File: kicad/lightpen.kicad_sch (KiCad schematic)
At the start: 4 parts, among them J16 Light Pen, U141 74LS74, U89 74LS04

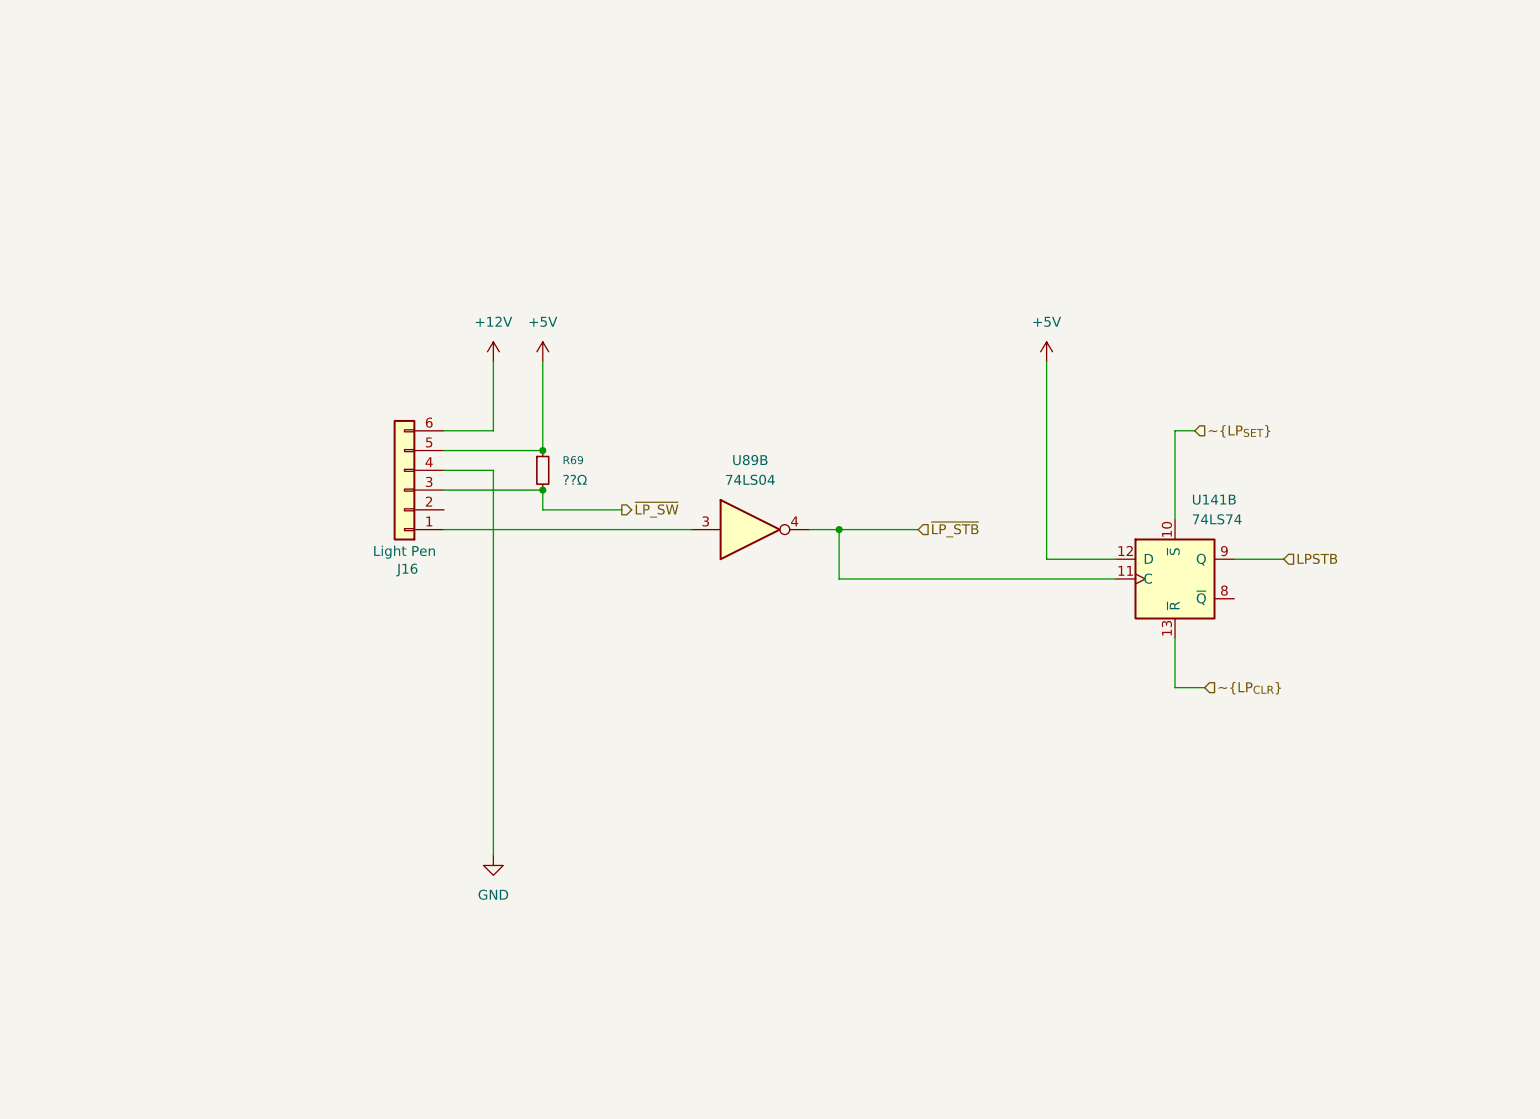
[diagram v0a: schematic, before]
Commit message: More updates
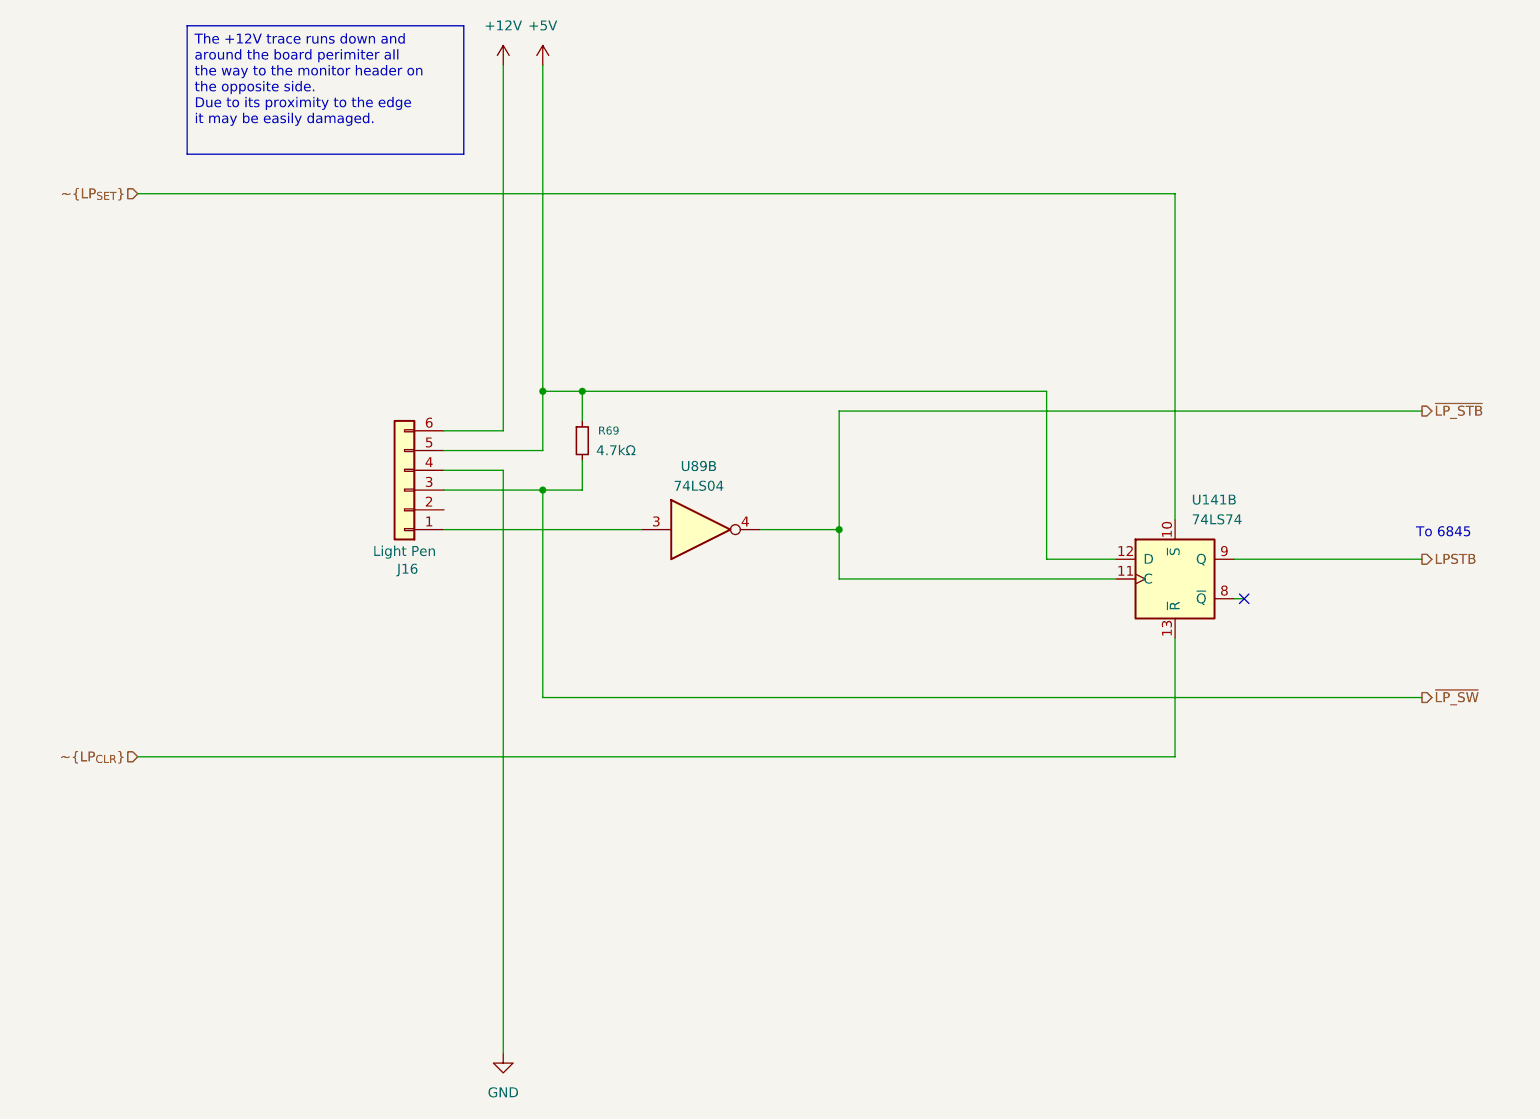
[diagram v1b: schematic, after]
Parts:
- R69: value ??Ω -> 4.7kΩ; seq_notes (none) -> Yellow, Violet, Red, Gold
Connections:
- no-connect marks 0 -> 1
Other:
- note added: "To 6845"
- title: (none) -> Video Unit: Light Pen Header
- moved on the sheet: R69, U89B
